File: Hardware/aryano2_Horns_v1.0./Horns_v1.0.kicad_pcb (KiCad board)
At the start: 2 copper layers, 39.8 x 37.3 mm, 17 parts, among them J1 Conn_01x02_Female, J2 Conn_01x03_Female, J3 Conn_01x02_Female, J4 Conn_01x02_Female, Q1 IRLIZ44N

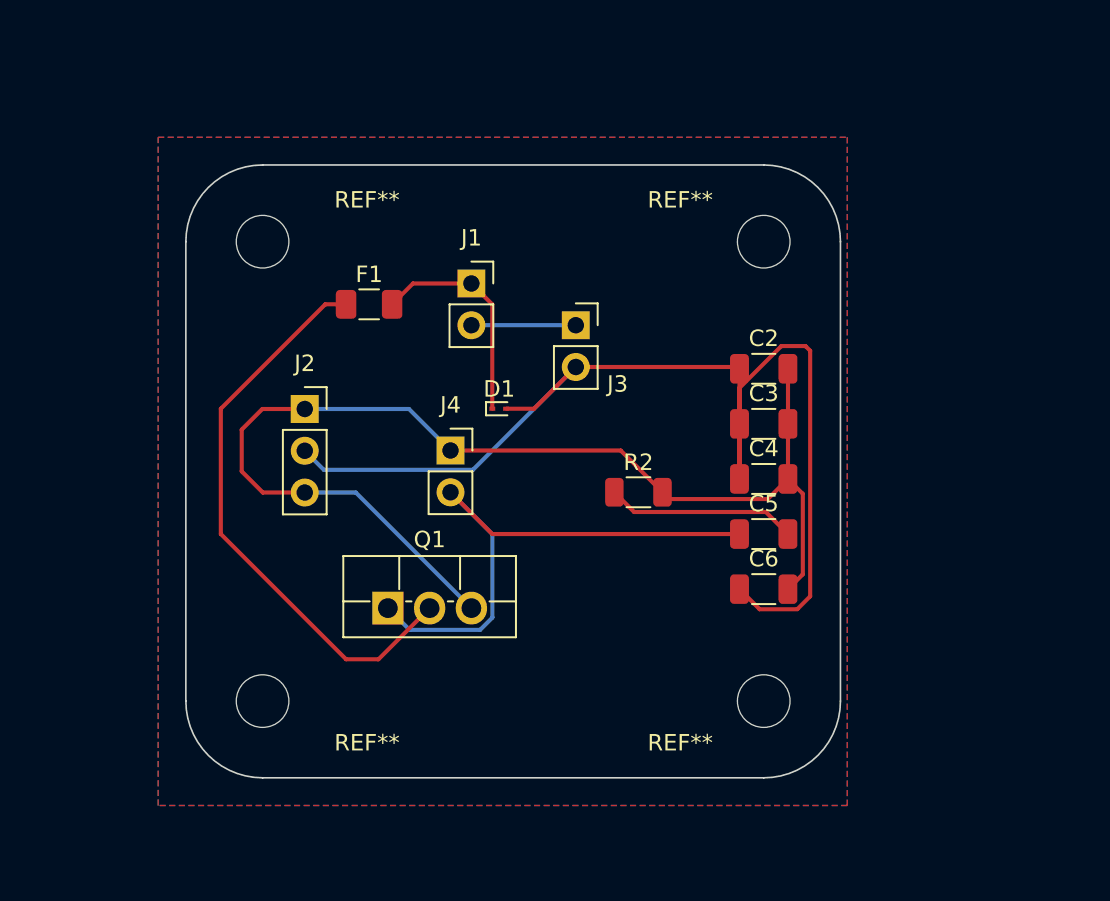
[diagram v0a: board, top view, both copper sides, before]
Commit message: final , finished hardware project 2
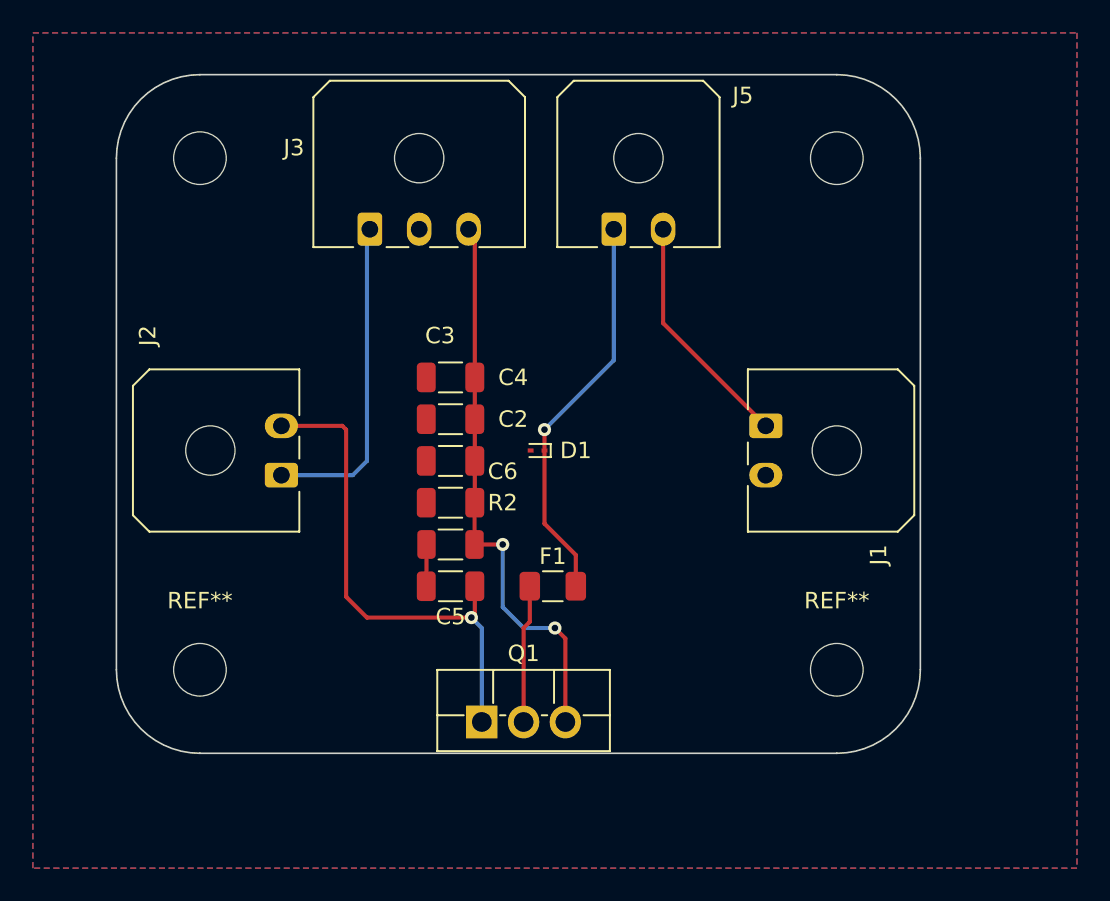
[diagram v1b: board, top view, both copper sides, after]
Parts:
- removed J4: Conn_01x02_Female, Connector_PinSocket_2.54mm:PinSocket_1x02_P2.54mm_Vertical
- removed the REF** at (124.5, 118.1)
- removed the REF** at (94.0, 118.1)
- removed the REF** at (94.0, 90.2)
- removed the REF** at (124.5, 90.2)
- added J5: Conn_01x02, Connector_Molex:Molex_Micro-Fit_3.0_43650-0200_1x02_P3.00mm_Horizontal, F.Cu at (115.3, 89.4)
- added REF**: MountingHole_3.2mm_M3, MountingHole:MountingHole_3.2mm_M3, F.Cu at (90.2, 85.1)
- added REF**: MountingHole_3.2mm_M3, MountingHole:MountingHole_3.2mm_M3, F.Cu at (128.9, 116.2)
- added REF**: MountingHole_3.2mm_M3, MountingHole:MountingHole_3.2mm_M3, F.Cu at (128.9, 85.1)
- added REF**: MountingHole_3.2mm_M3, MountingHole:MountingHole_3.2mm_M3, F.Cu at (90.2, 116.2)
- J1: value Conn_01x02_Female -> Conn_01x02; footprint Connector_PinSocket_2.54mm:PinSocket_1x02_P2.54mm_Vertical -> Connector_Molex:Molex_Micro-Fit_3.0_43650-0200_1x02_P3.00mm_Horizontal
- J2: value Conn_01x03_Female -> Conn_01x02; footprint Connector_PinSocket_2.54mm:PinSocket_1x03_P2.54mm_Vertical -> Connector_Molex:Molex_Micro-Fit_3.0_43650-0200_1x02_P3.00mm_Horizontal
- J3: value Conn_01x02_Female -> Conn_01x03; footprint Connector_PinSocket_2.54mm:PinSocket_1x02_P2.54mm_Vertical -> Connector_Molex:Molex_Micro-Fit_3.0_43650-0300_1x03_P3.00mm_Horizontal
- moved F1 20.5 mm to (111.6, 111.1)
- moved J1 19.9 mm to (124.6, 101.4), turned to -90 degrees
- moved C2 19.9 mm to (105.4, 103.5)
- moved C6 19.8 mm to (105.4, 106.0)
- moved C4 19.4 mm to (105.4, 101.0)
- moved C5 19.3 mm to (105.4, 111.1), turned to 180 degrees
- moved C3 19.3 mm to (105.4, 98.4)
- moved J3 13.8 mm to (100.5, 89.4)
- moved R2 11.9 mm to (105.4, 108.6)
- moved Q1 8.98 mm to (107.3, 119.4)
- moved J2 4.27 mm to (95.1, 104.4), turned to 90 degrees
- moved D1 3.45 mm to (110.7, 102.9), turned to 180 degrees
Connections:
- J1 pad 1: /HORN_IN -> Net-(J1-Pin_1)
- J1 pad 2: Net-(J1-Pin_2) -> +24V
- J2 pad 2: +24V -> /HORN_CTRL
- J3 pad 1: Net-(J1-Pin_2) -> GND
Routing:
- net +24V: track 72.6 -> 0.00 mm
- net Net-(Q1-D): track 35.0 -> 8.41 mm
- net GND: track 70.7 -> 54.3 mm, vias 0 -> 2
- net Net-(J1-Pin_1): track 0.00 -> 14.9 mm
- net /HORN_IN: track 13.5 -> 24.2 mm, vias 0 -> 1
- net Net-(C5-Pad2): track 11.6 -> 2.55 mm
- net Net-(J1-Pin_2): track 6.35 -> 0.00 mm
- net /HORN_CTRL: track 34.5 -> 30.9 mm, vias 0 -> 1
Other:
- board size 39.8 x 37.3 mm -> 48.9 x 41.3 mm
